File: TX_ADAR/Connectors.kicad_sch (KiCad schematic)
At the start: 10 parts, among them J1 Conn_Coaxial, J11 RJ45_LED_Shielded, J12 RJ45_LED_Shielded, J13 Conn_Coaxial, J14 Conn_Coaxial, J15 FX8-120S-SV21, J16 RJ45_LED_Shielded, J17 Conn_Coaxial, J18 Conn_Coaxial, J2 Conn_Coaxial

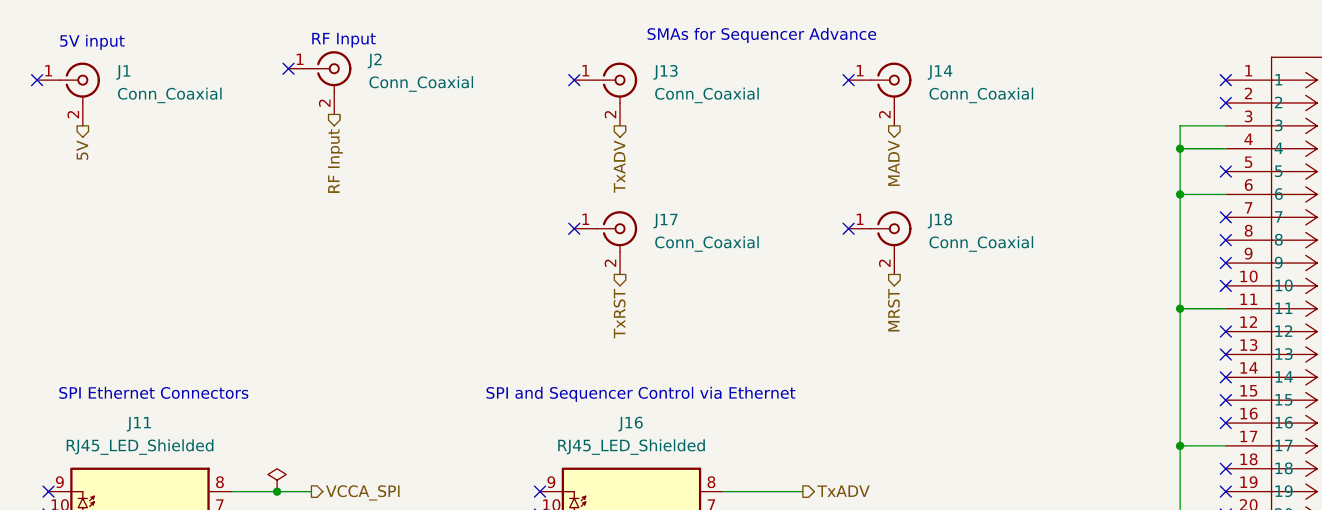
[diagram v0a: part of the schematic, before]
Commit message: Fixing problems pointed out
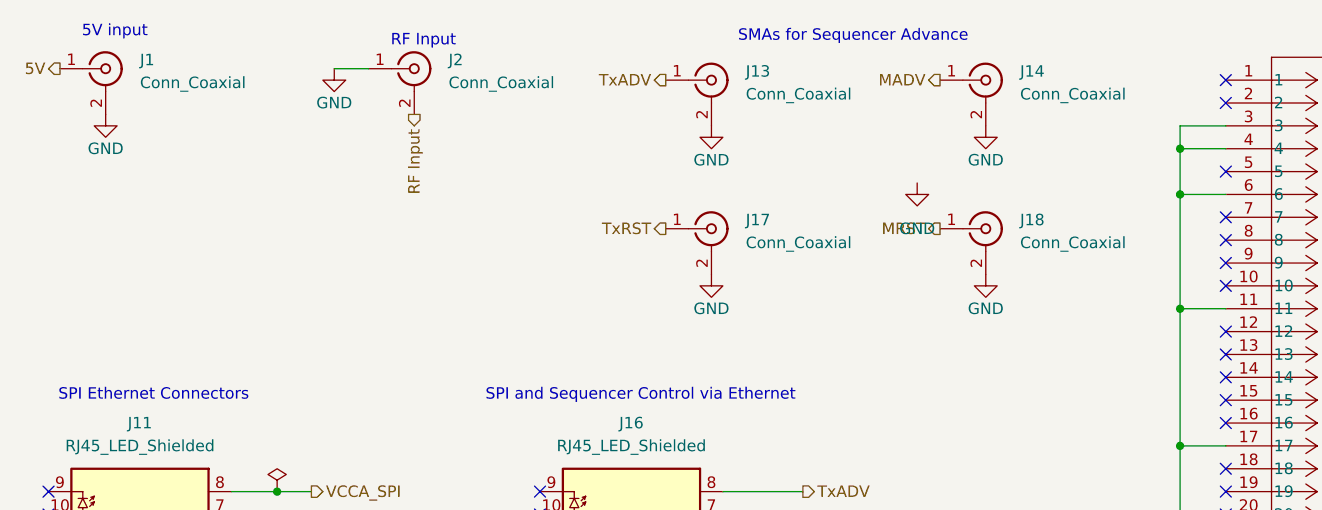
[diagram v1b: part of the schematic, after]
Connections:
- net 5V: now also J1.1 (In); no longer J1.2 (Ext)
- net GND: now also J1.2 (Ext), J13.2 (Ext), J14.2 (Ext), J17.2 (Ext), J18.2 (Ext), J2.1 (In)
- net MADV: now also J14.1 (In); no longer J14.2 (Ext)
- net MRST: now also J18.1 (In); no longer J18.2 (Ext)
- net TxADV: now also J13.1 (In); no longer J13.2 (Ext)
- net TxRST: now also J17.1 (In); no longer J17.2 (Ext)
- no-connect marks 105 -> 99
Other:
- moved on the sheet: J1, J13, J14, J17, J18, J2
